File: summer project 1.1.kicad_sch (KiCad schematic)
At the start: 11 parts, among them J4 Conn_01x02_Socket, J5 Conn_01x02_Socket, J6 Screw_Terminal_01x02, Q3 NMOS, Q4 NMOS, U3 LM5050-1_mod2, U4 LM5050-1_mod2

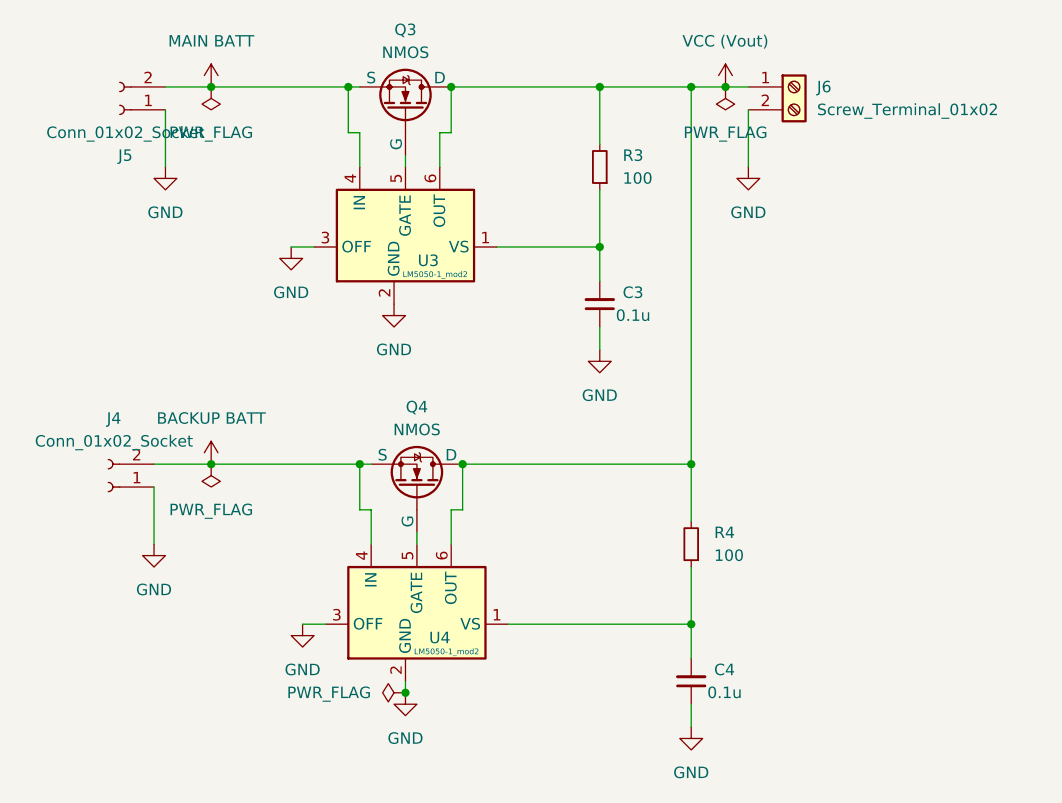
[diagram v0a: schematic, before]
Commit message: symbol design
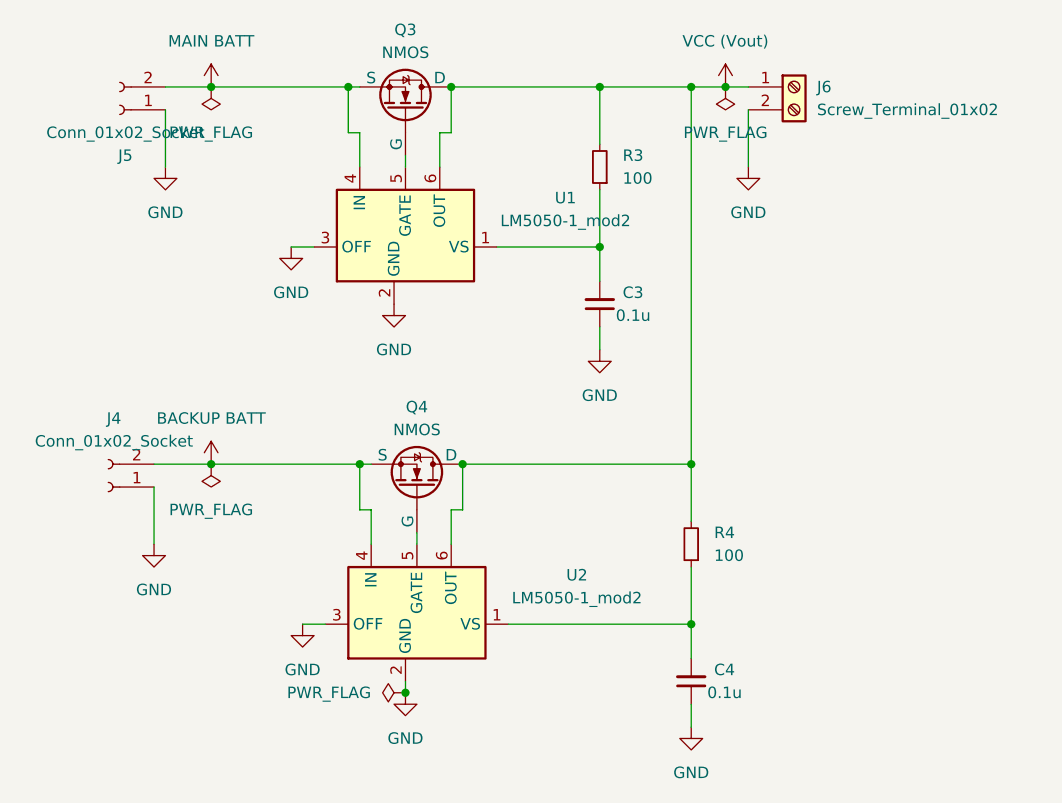
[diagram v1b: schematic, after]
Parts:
- removed U3, U4: LM5050-1_mod2, Package_TO_SOT_SMD:TSOT-23-6, symbol smp 1:LM5050-1_mod2
- added U1, U2: LM5050-1_mod2, Package_TO_SOT_SMD:TSOT-23-6, symbol smp1:LM5050-1_mod2
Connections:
- net BACKUP BATT: now also U2.4 (IN)
- net GND: now also U1.2 (GND), U1.3 (OFF), U2.2 (GND), U2.3 (OFF)
- net MAIN BATT: now also U1.4 (IN)
- net VCC (Vout): now also U1.6 (OUT), U2.6 (OUT)
- net at C3.2, R3.1: now also U1.1 (VS)
- net at C4.2, R4.1: now also U2.1 (VS)
- net at Q4.2 (G): now also U2.5 (GATE)
- net at Q3.2 (G): now also U1.5 (GATE)
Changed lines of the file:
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@@
-	)
-	(symbol
-		(lib_id "smp 1:LM5050-1_mod2")
-		(at 138.43 114.3 90)
-		(unit 1)
-		(exclude_from_sim no)
-		(in_bom yes)
-		(on_board yes)
-		(dnp no)
-		(property "Reference" "U4"
-			(at 140.97 117.094 90)
-			(effects
-				(font
-					(size 1.27 1.27)
-				)
-			)
-		)
-		(property "Value" "LM5050-1_mod2"
-			(at 141.732 118.618 90)
-			(effects
-				(font
-					(size 0.635 0.635)
-				)
-			)
-		)
-		(property "Footprint" "Package_TO_SOT_SMD:TSOT-23-6"
-			(at 147.32 97.79 0)
-			(effects
-				(font
-					(size 1.27 1.27)
-				)
-				(hide yes)
-			)
-		)
-		(property "Datasheet" "http://www.ti.com/lit/ds/symlink/lm5050-1-q1.pdf"
-			(at 139.7 86.36 0)
-			(effects
-				(font
-					(size 1.27 1.27)
-				)
-				(hide yes)
-			)
-		)
-		(property "Description" "High side OR-ing FET controller, 5V to 75V operation, TSOT-23-6"
-			(at 138.43 114.3 0)
-			(effects
-				(font
-					(size 1.27 1.27)
-				)
-				(hide yes)
-			)
-		)
-		(pin "5"
-		)
-		(pin "1"
-		)
-		(pin "6"
-		)
-		(pin "4"
-		)
-		(pin "2"
-		)
-		(pin "3"
-		)
-		(instances
-			(project "summer project 1.1"
-				(path "/19e44473-05a8-487a-9fcb-12427ac5e96b"
-					(reference "U4")
-					(unit 1)
-				)
-			)
-		)
-	)
-	(symbol
-		(lib_id "smp 1:LM5050-1_mod2")
-		(at 137.16 72.39 90)
-		(unit 1)
-		(exclude_from_sim no)
-		(in_bom yes)
-		(on_board yes)
-		(dnp no)
-		(property "Reference" "U3"
-			(at 139.7 75.184 90)
-			(effects
-				(font
-					(size 1.27 1.27)
-				)
-			)
-		)
-		(property "Value" "LM5050-1_mod2"
-			(at 140.462 76.708 90)
-			(effects
-				(font
-					(size 0.635 0.635)
-				)
-			)
-		)
-		(property "Footprint" "Package_TO_SOT_SMD:TSOT-23-6"
-			(at 146.05 55.88 0)
-			(effects
-				(font
-					(size 1.27 1.27)
-				)
-				(hide yes)
-			)
-		)
-		(property "Datasheet" "http://www.ti.com/lit/ds/symlink/lm5050-1-q1.pdf"
-			(at 138.43 44.45 0)
-			(effects
-				(font
-					(size 1.27 1.27)
-				)
-				(hide yes)
-			)
-		)
-		(property "Description" "High side OR-ing FET controller, 5V to 75V operation, TSOT-23-6"
-			(at 137.16 72.39 0)
-			(effects
-				(font
-					(size 1.27 1.27)
-				)
-				(hide yes)
-			)
-		)
-		(pin "5"
-		)
-		(pin "1"
-		)
-		(pin "6"
-		)
-		(pin "4"
-		)
-		(pin "2"
-		)
-		(pin "3"
-		)
-		(instances
-			(project "summer project 1.1"
-				(path "/19e44473-05a8-487a-9fcb-12427ac5e96b"
-					(reference "U3")
-					(unit 1)
-				)
-			)
-		)
 	)
 	(symbol
@@
 	)
 	(symbol
+		(lib_id "smp1:LM5050-1_mod2")
+		(at 138.43 114.3 90)
+		(unit 1)
+		(exclude_from_sim no)
+		(in_bom yes)
+		(on_board yes)
+		(dnp no)
+		(fields_autoplaced yes)
+		(property "Reference" "U2"
+			(at 156.21 110.1246 90)
+			(effects
+				(font
+					(size 1.27 1.27)
+				)
+			)
+		)
+		(property "Value" "LM5050-1_mod2"
+			(at 156.21 112.6646 90)
+			(effects
+				(font
+					(size 1.27 1.27)
+				)
+			)
+		)
+		(property "Footprint" "Package_TO_SOT_SMD:TSOT-23-6"
+			(at 147.32 97.79 0)
+			(effects
+				(font
+					(size 1.27 1.27)
+				)
+				(hide yes)
+			)
+		)
+		(property "Datasheet" "http://www.ti.com/lit/ds/symlink/lm5050-1-q1.pdf"
+			(at 139.7 86.36 0)
+			(effects
+				(font
+					(size 1.27 1.27)
+				)
+				(hide yes)
+			)
+		)
+		(property "Description" "High side OR-ing FET controller, 5V to 75V operation, TSOT-23-6"
+			(at 138.43 114.3 0)
+			(effects
+				(font
+					(size 1.27 1.27)
+				)
+				(hide yes)
+			)
+		)
+		(pin "6"
+		)
+		(pin "5"
+		)
+		(pin "2"
+		)
+		(pin "1"
+		)
+		(pin "3"
+		)
+		(pin "4"
+		)
+		(instances
+			(project "summer project 1.1"
+				(path "/19e44473-05a8-487a-9fcb-12427ac5e96b"
+					(reference "U2")
+					(unit 1)
+				)
+			)
+		)
+	)
+	(symbol
 		(lib_id "power:GND")
 		(at 175.26 64.77 0)
@@
 					(unit 1)
 				)
+			)
+		)
+	)
+	(symbol
+		(lib_id "smp1:LM5050-1_mod2")
+		(at 137.16 72.39 90)
+		(unit 1)
+		(exclude_from_sim no)
+		(in_bom yes)
+		(on_board yes)
+		(dnp no)
+		(fields_autoplaced yes)
+		(property "Reference" "U1"
+			(at 154.94 68.2146 90)
+			(effects
+				(font
+					(size 1.27 1.27)
+				)
+			)
+		)
+		(property "Value" "LM5050-1_mod2"
+			(at 154.94 70.7546 90)
+			(effects
+				(font
+					(size 1.27 1.27)
+				)
+			)
+		)
+		(property "Footprint" "Package_TO_SOT_SMD:TSOT-23-6"
+			(at 146.05 55.88 0)
+			(effects
+				(font
+					(size 1.27 1.27)
+				)
+				(hide yes)
+			)
+		)
+		(property "Datasheet" "http://www.ti.com/lit/ds/symlink/lm5050-1-q1.pdf"
+			(at 138.43 44.45 0)
+			(effects
+				(font
+					(size 1.27 1.27)
+				)
+				(hide yes)
+			)
+		)
+		(property "Description" "High side OR-ing FET controller, 5V to 75V operation, TSOT-23-6"
+			(at 137.16 72.39 0)
+			(effects
+				(font
+					(size 1.27 1.27)
+				)
+				(hide yes)
+			)
+		)
+		(pin "6"
+		)
+		(pin "5"
+		)
+		(pin "2"
+		)
+		(pin "1"
+		)
+		(pin "3"
+		)
+		(pin "4"
+		)
+		(instances
+			(project ""
+				(path "/19e44473-05a8-487a-9fcb-12427ac5e96b"
+					(reference "U1")
+					(unit 1)
+				)
